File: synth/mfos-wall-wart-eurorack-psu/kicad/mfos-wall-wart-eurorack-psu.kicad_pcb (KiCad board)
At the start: 2 copper layers, 80 x 100 mm, 50 parts, among them J1 JST-5, J2 TERMINAL-4, M1 MountingHole_3.2mm_M3_Pad, M2 MountingHole_3.2mm_M3_Pad, M3 MountingHole_3.2mm_M3_Pad, M4 MountingHole_3.2mm_M3_Pad, U1 L7805CV, U2 L7812CV, U3 L7912CV

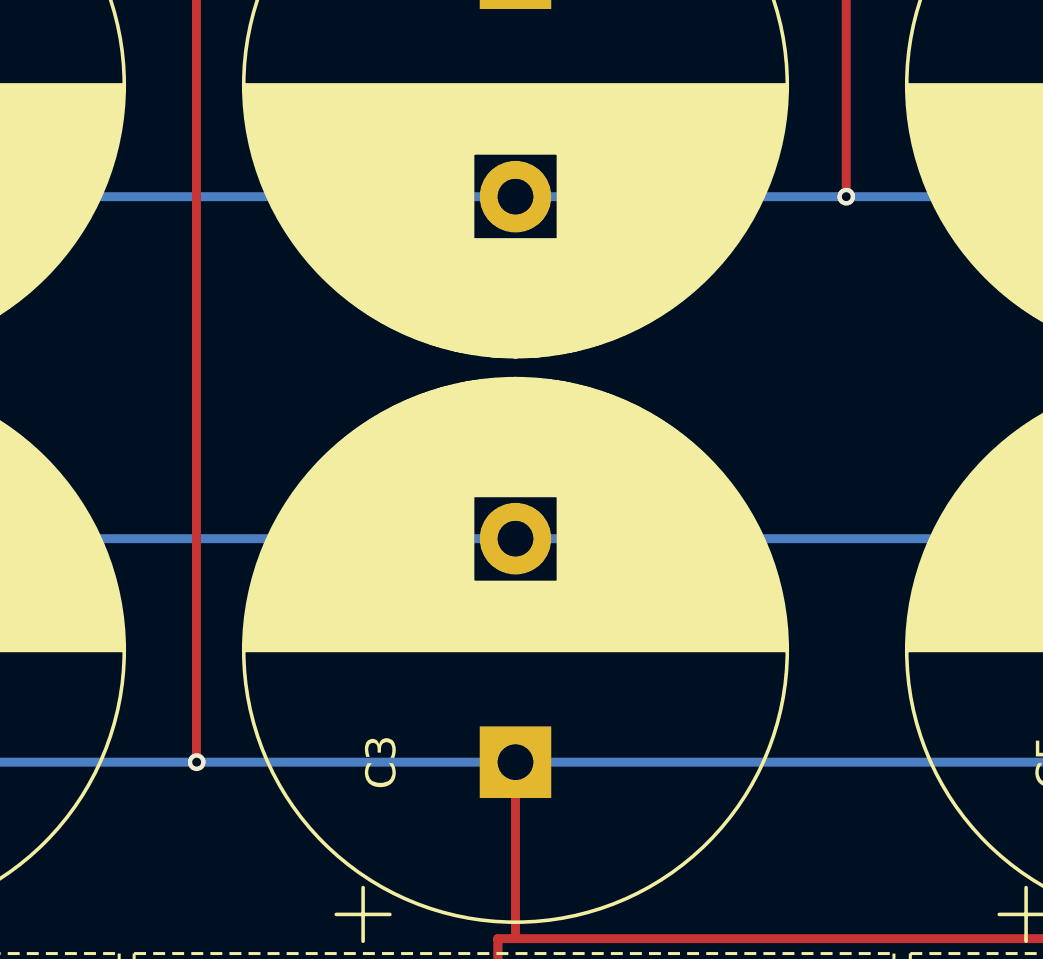
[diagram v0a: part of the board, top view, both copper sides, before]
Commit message: prototyping board
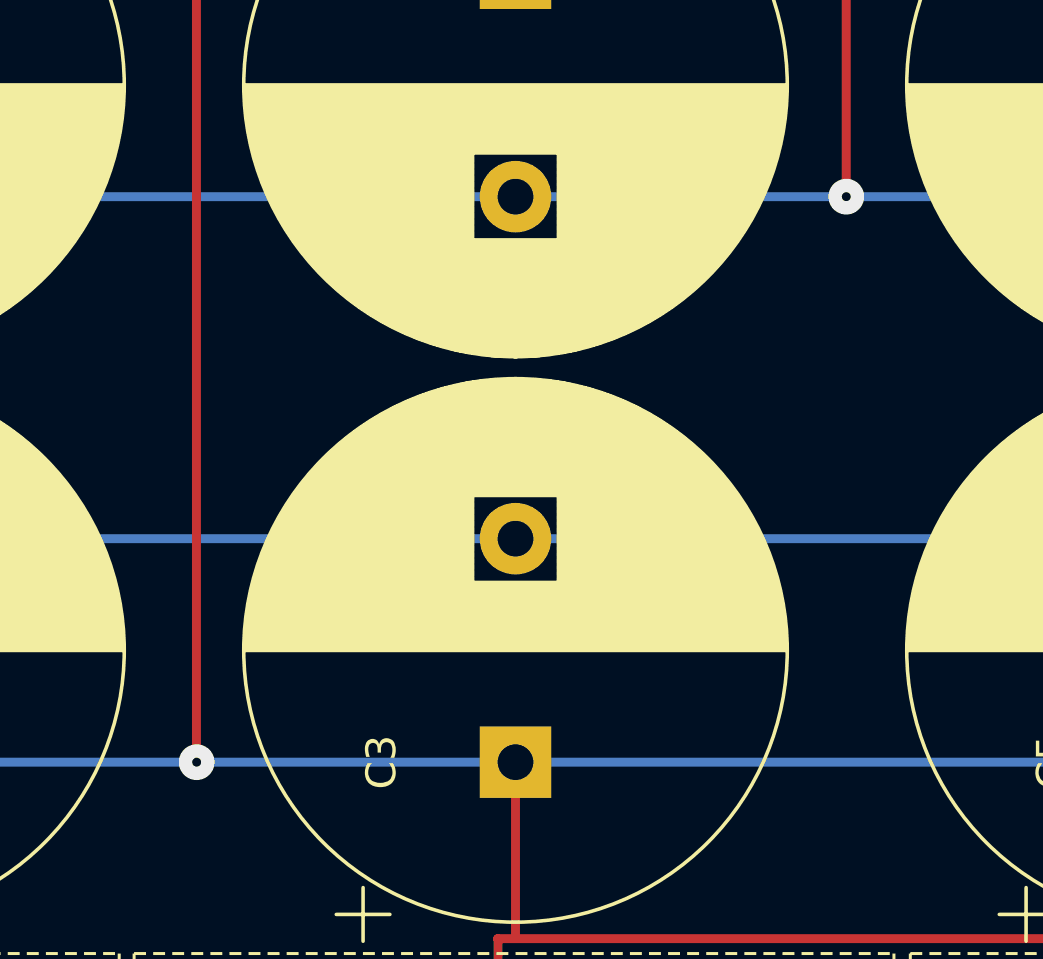
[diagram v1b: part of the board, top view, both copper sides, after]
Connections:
- net Net-(D1-K) renamed 12VAC
